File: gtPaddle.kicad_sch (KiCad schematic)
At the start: 40 parts, among them IC1 74157N, IC2 74157N, J1 Conn_01x02_Pin, J2 Conn_01x02_Pin, J3 Conn_01x02_Pin, J4 Conn_01x02_Pin, Q1 2N3904, Q10 2N3904, Q2 2N3904, Q3 2N3904, Q9 2N3904, U1 ADC0804LCN

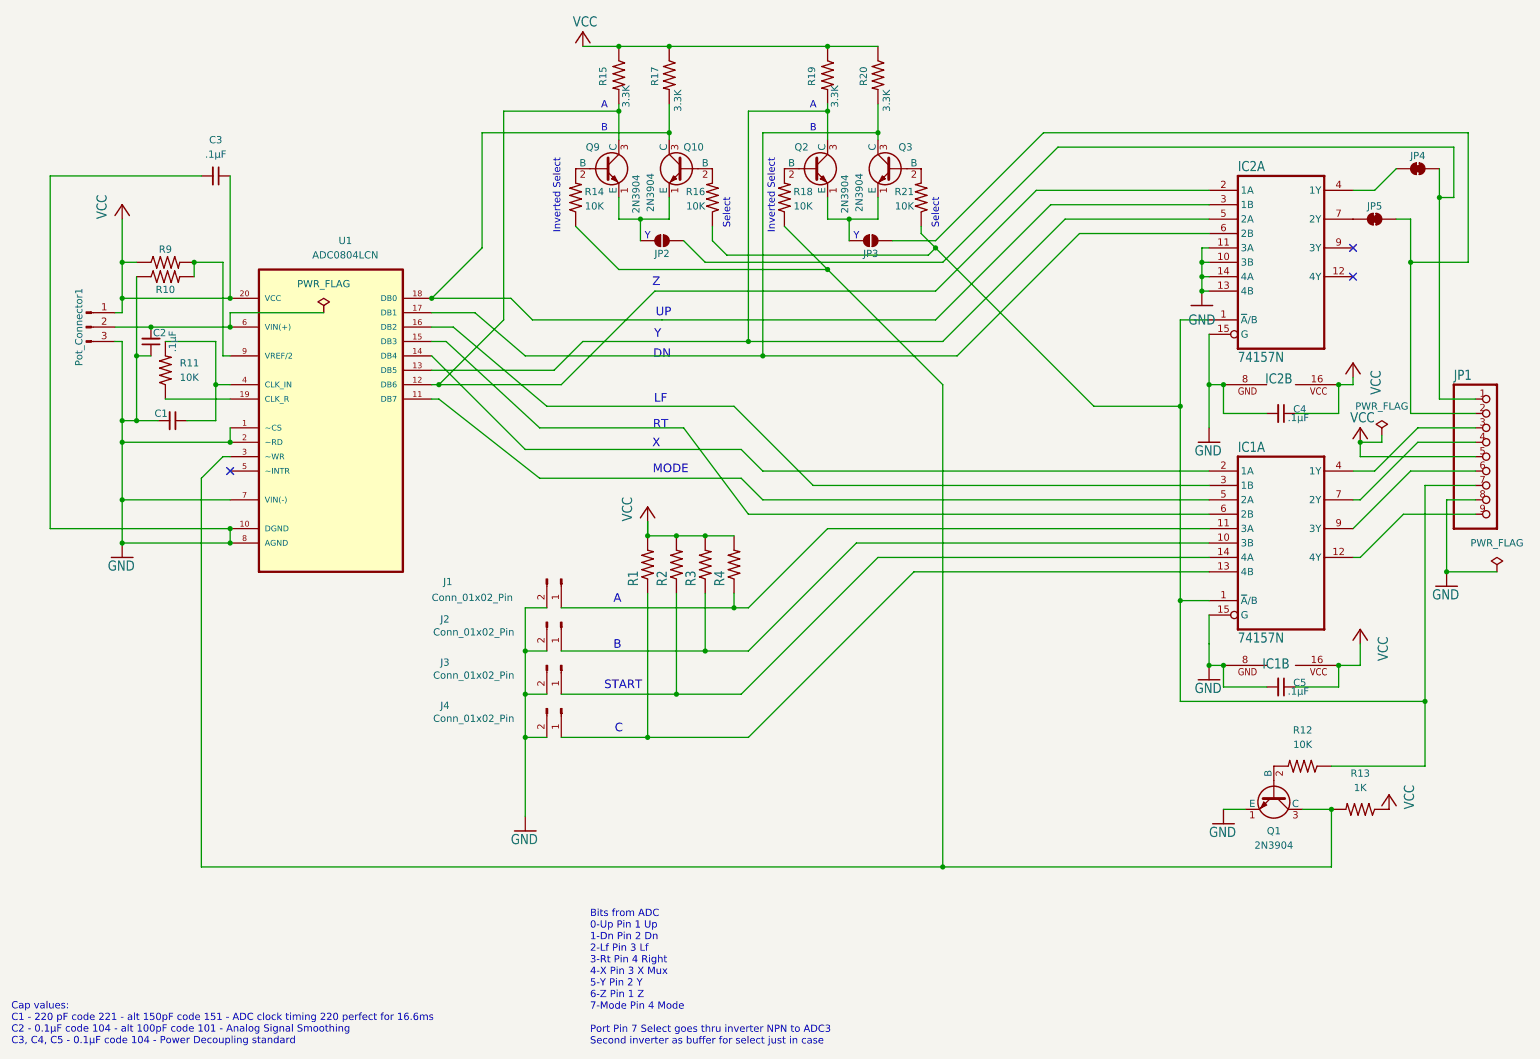
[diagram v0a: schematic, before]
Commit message: remove npn muxes
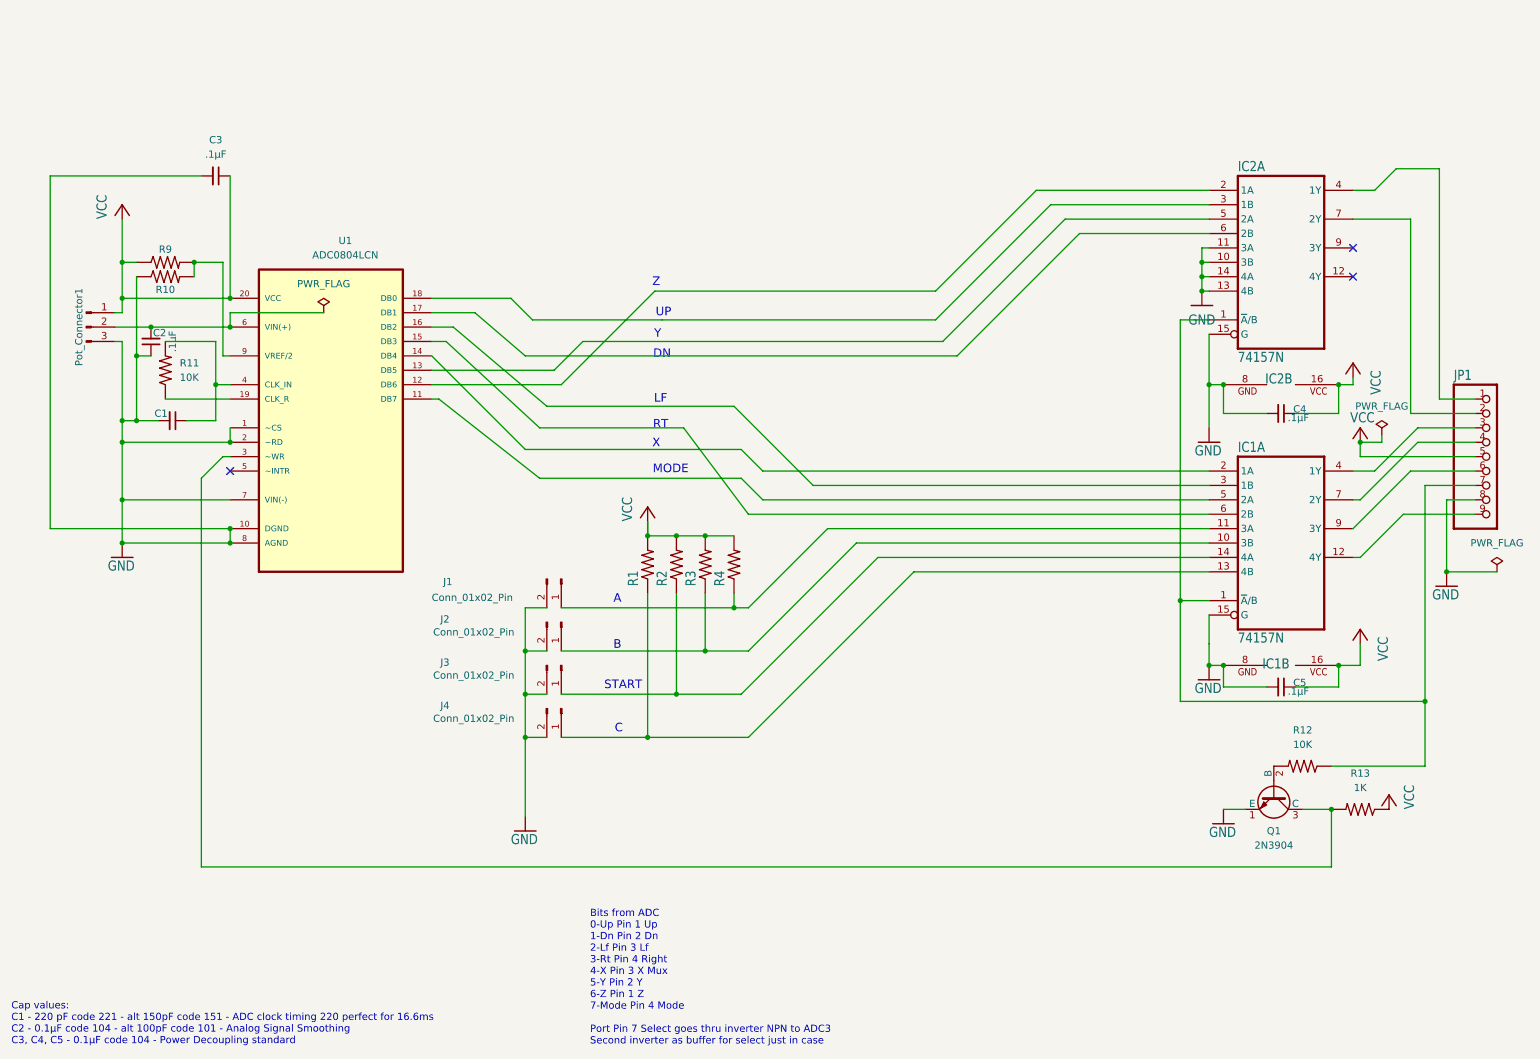
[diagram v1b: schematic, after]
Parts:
- removed JP2, JP3: SolderJumper_2_Open, Jumper:SolderJumper-2_P1.3mm_Open_RoundedPad1.0x1.5mm, symbol Jumper:SolderJumper_2_Open
- removed JP4, JP5: SolderJumper_2_Bridged, Jumper:SolderJumper-2_P1.3mm_Bridged_RoundedPad1.0x1.5mm, symbol Jumper:SolderJumper_2_Bridged
- removed Q10, Q2, Q3, Q9: 2N3904, Package_TO_SOT_THT:TO-92S-EBC, symbol Transistor_BJT:2N3904
- removed R14, R16, R18, R21: 10K, Resistor_THT:R_Axial_DIN0309_L9.0mm_D3.2mm_P2.54mm_Vertical, symbol gpad1-eagle-import:R-US_0207/10
- removed R15, R17, R19, R20: 3.3K, Resistor_THT:R_Axial_DIN0309_L9.0mm_D3.2mm_P2.54mm_Vertical, symbol gpad1-eagle-import:R-US_0207/10
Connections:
- net at IC2.4 (1Y): now also JP1.1
- net at JP1.2: now also IC2.7 (2Y)
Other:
- note removed: "Inverted Select"
- note removed: "Select"
